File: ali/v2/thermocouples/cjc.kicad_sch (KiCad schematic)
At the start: 23 parts, among them U10 TMP117AIDRVR, U11 TMP117AIDRVR, U12 TMP117AIDRVR, U13 TMP117AIDRVR, U7 TCA9543A, U8 TMP117AIDRVR, U9 TMP117AIDRVR

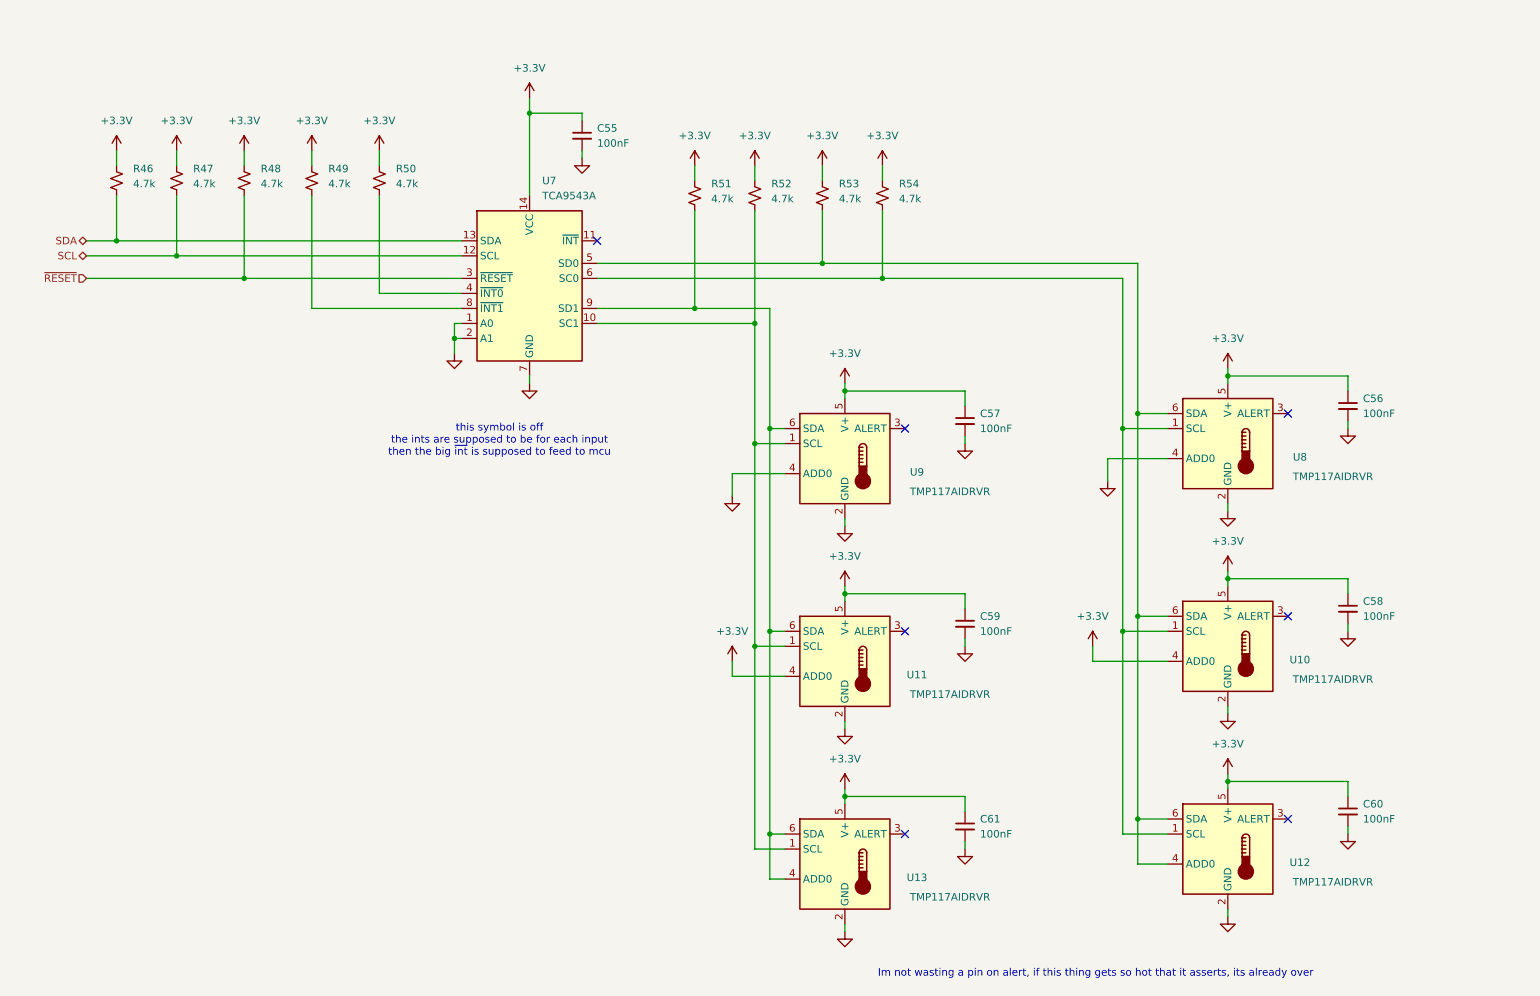
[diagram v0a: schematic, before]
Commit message: Small documentation
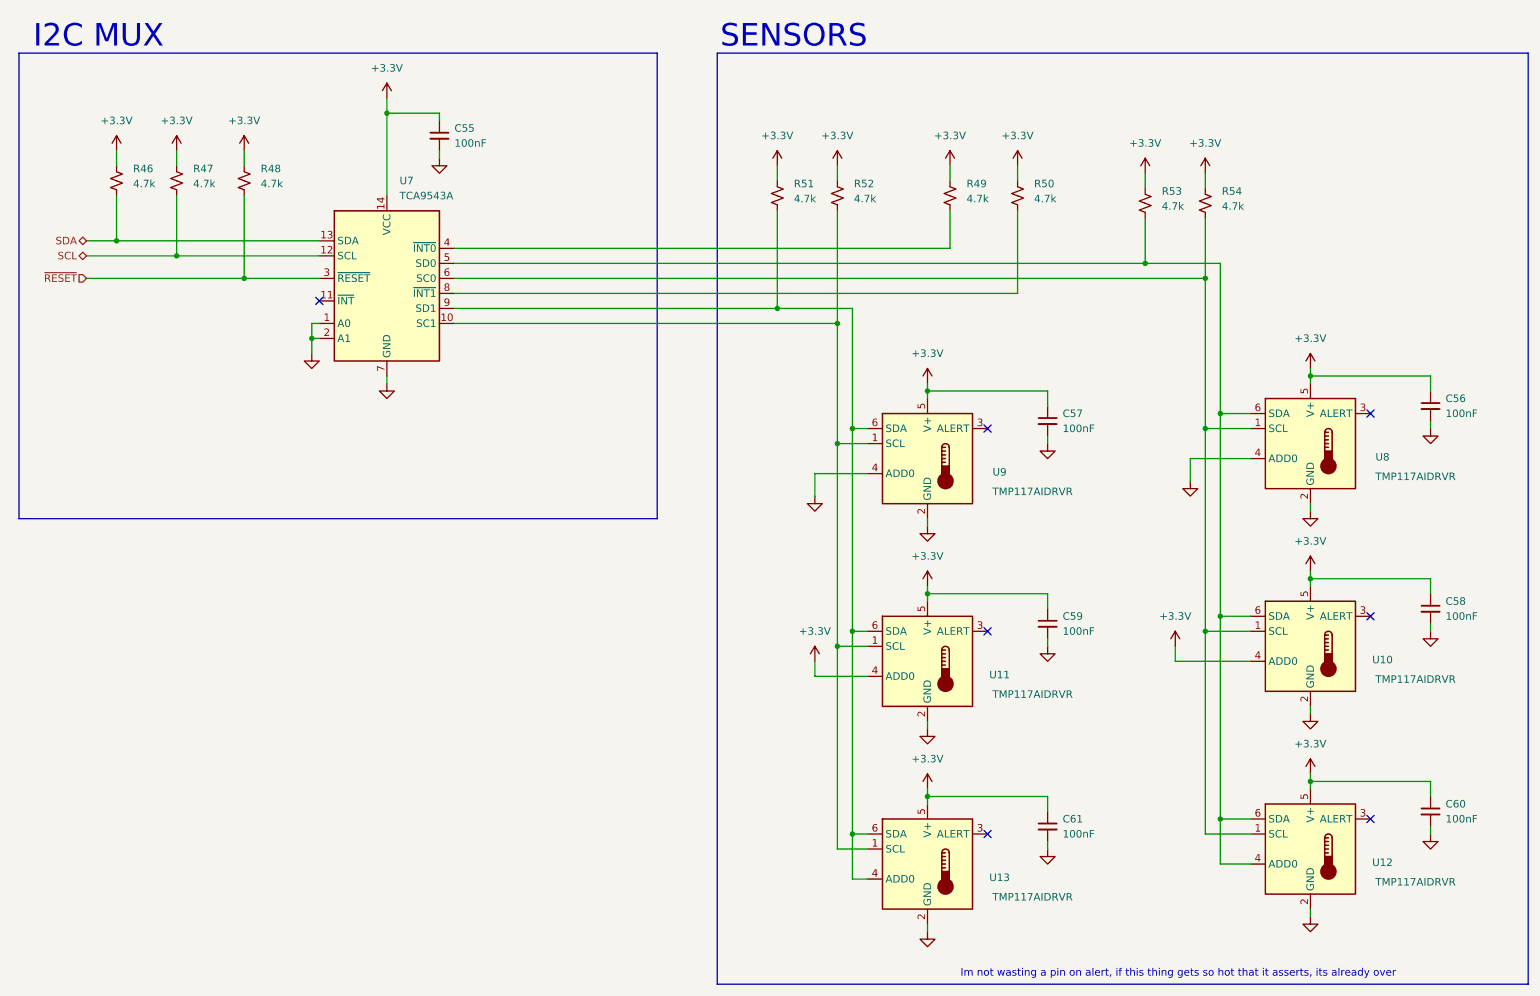
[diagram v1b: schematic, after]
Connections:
- net at R50.2: now also U7.8 (~{INT1}); no longer U7.4 (~{INT0})
- net at R49.2: now also U7.4 (~{INT0}); no longer U7.8 (~{INT1})
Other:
- note added: "I2C MUX"
- note added: "SENSORS"
- note removed: "this symbol is off the ints are supposed to be for each input then the big ~{int} is supposed to feed to mcu"
- moved on the sheet: C55, C56, C57, C58, C59, C60, C61, R51, R52, R53, R54, U10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
